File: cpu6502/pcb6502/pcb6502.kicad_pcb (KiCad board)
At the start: 2 copper layers, 134.6 x 96.5 mm, 39 parts, among them J1 Power, J2 RS232, J3 VIA PA, J4 VIA PB, J6 Address, J7 Data, J8 CPU, SW1 Reset, SW2 IRQ Enable, U1 6502, U2 EEPROM, U3 RAM, U4 65C22, U5 74HC00, U6 L7805, U7 W65C51NxP, U8 MAX232, U9 DS1813, X1 1MHz, Y1 Crystal

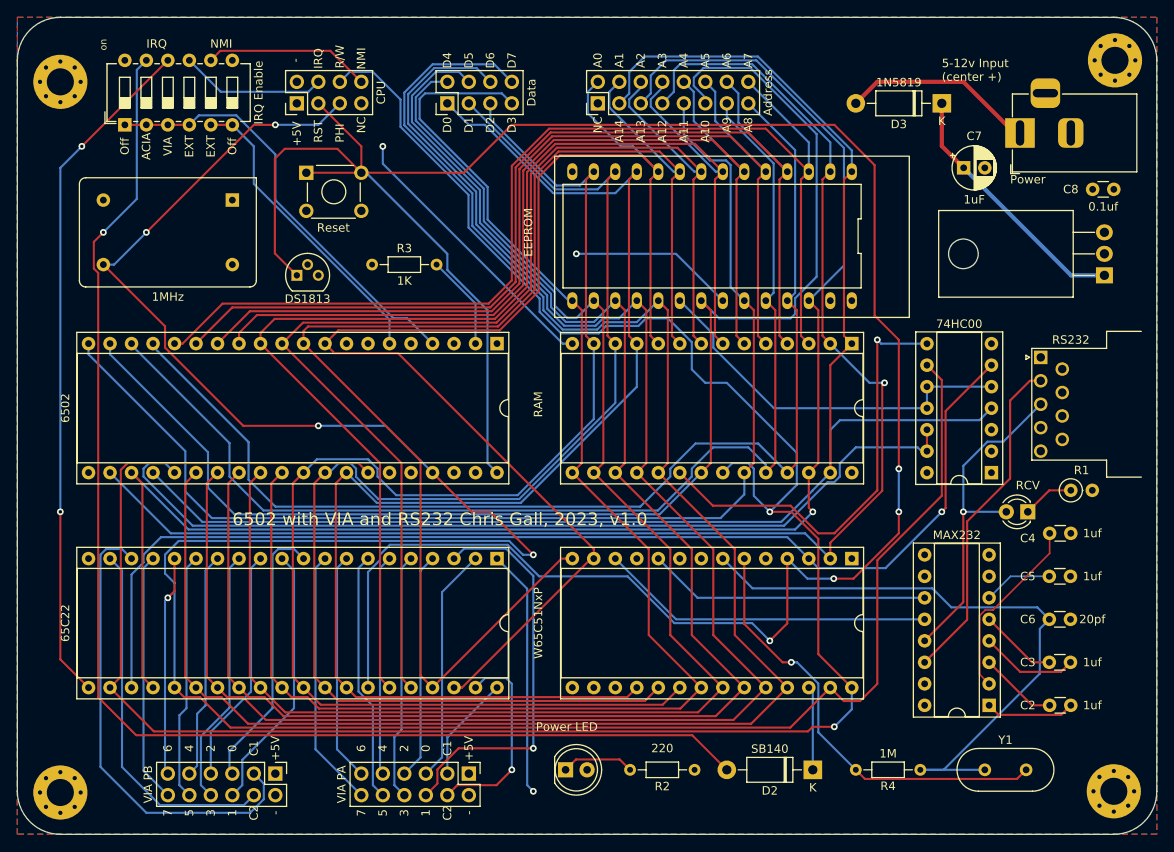
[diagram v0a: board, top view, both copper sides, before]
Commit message: tweaks
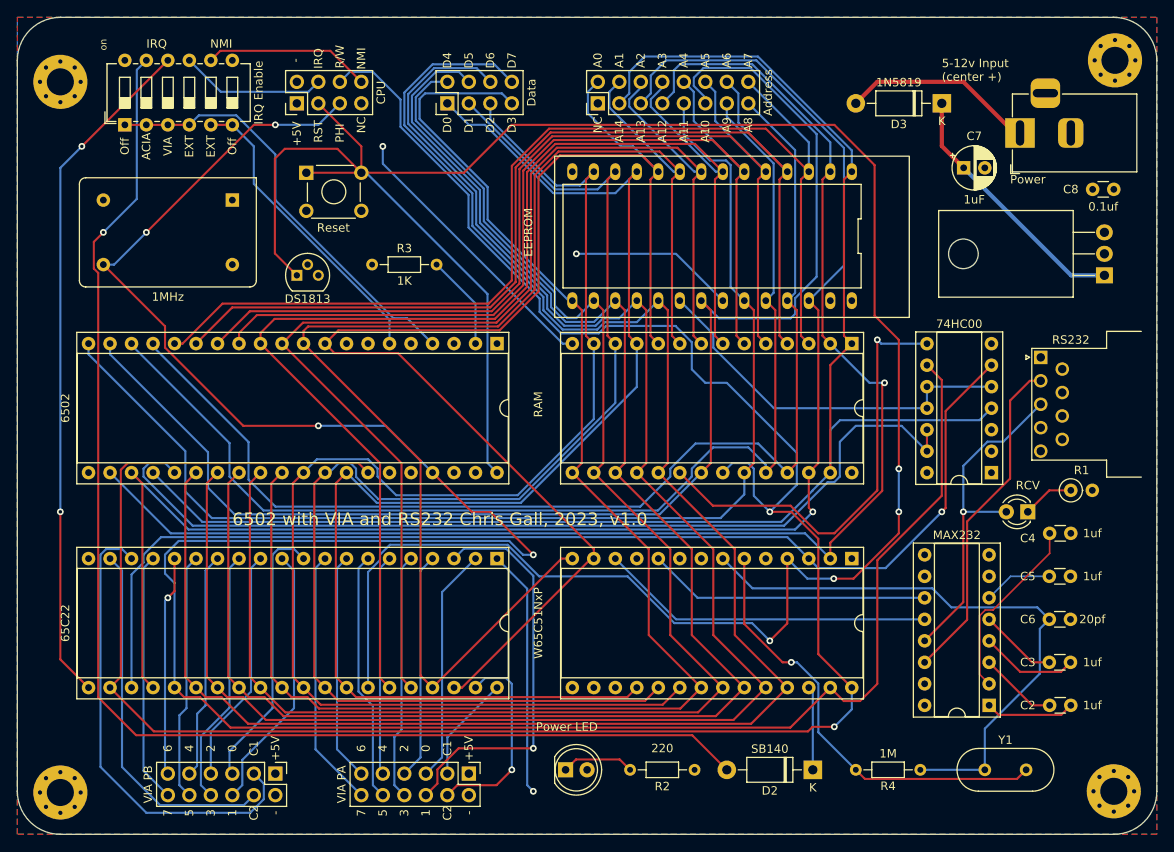
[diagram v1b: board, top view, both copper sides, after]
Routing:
- net /XTAL2: track 74.7 -> 70.1 mm
- net /A15: track 108.7 -> 111.4 mm
- net /R/W: track 276.1 -> 275.3 mm
